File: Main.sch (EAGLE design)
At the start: 47 parts, among them IC1 LM75A, IC2 ADUM1400, IC3 74LS14N, Q1 IRF9530, U1 L298, U2 LM 1084 IT5,0, U3 LM 1084 IT3,3, U4 L298, X1 Motors, X2 PIRs, X3 Battery, X4 Ultra Sonics

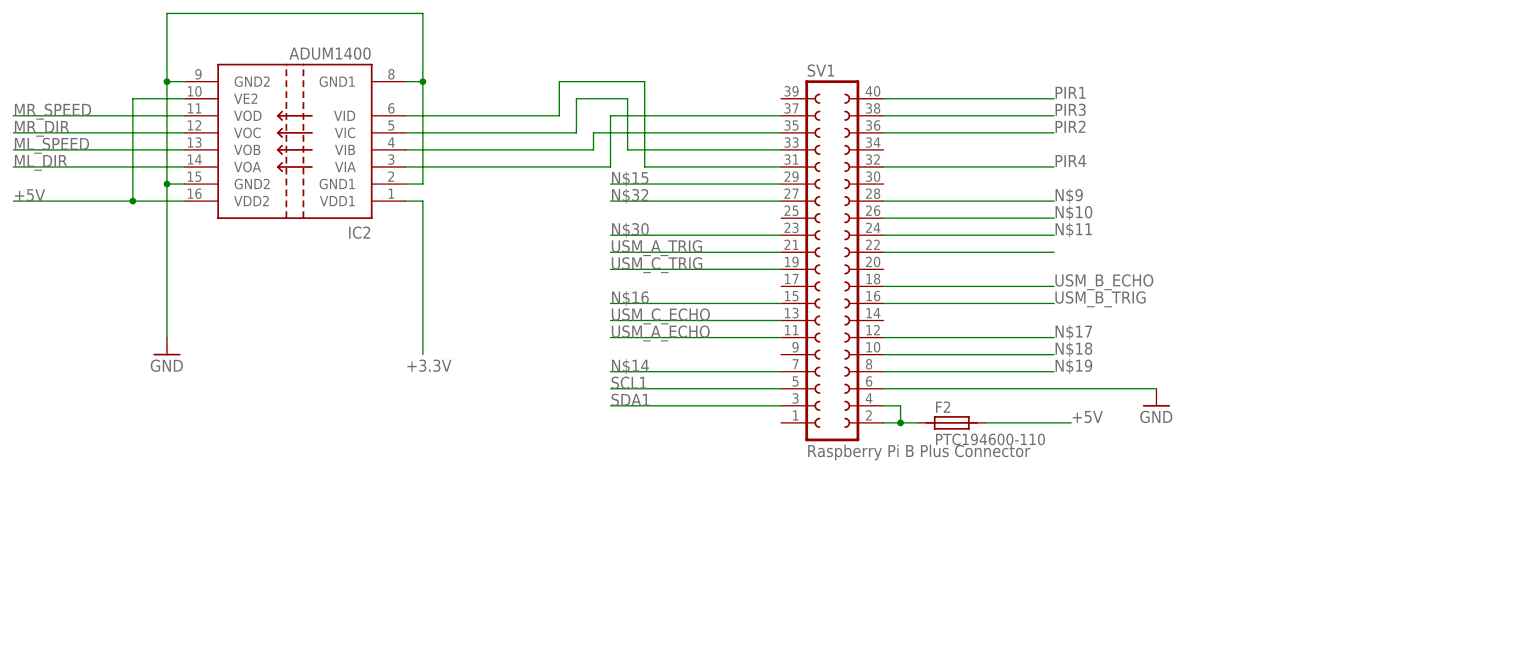
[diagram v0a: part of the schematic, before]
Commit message: playing with routes
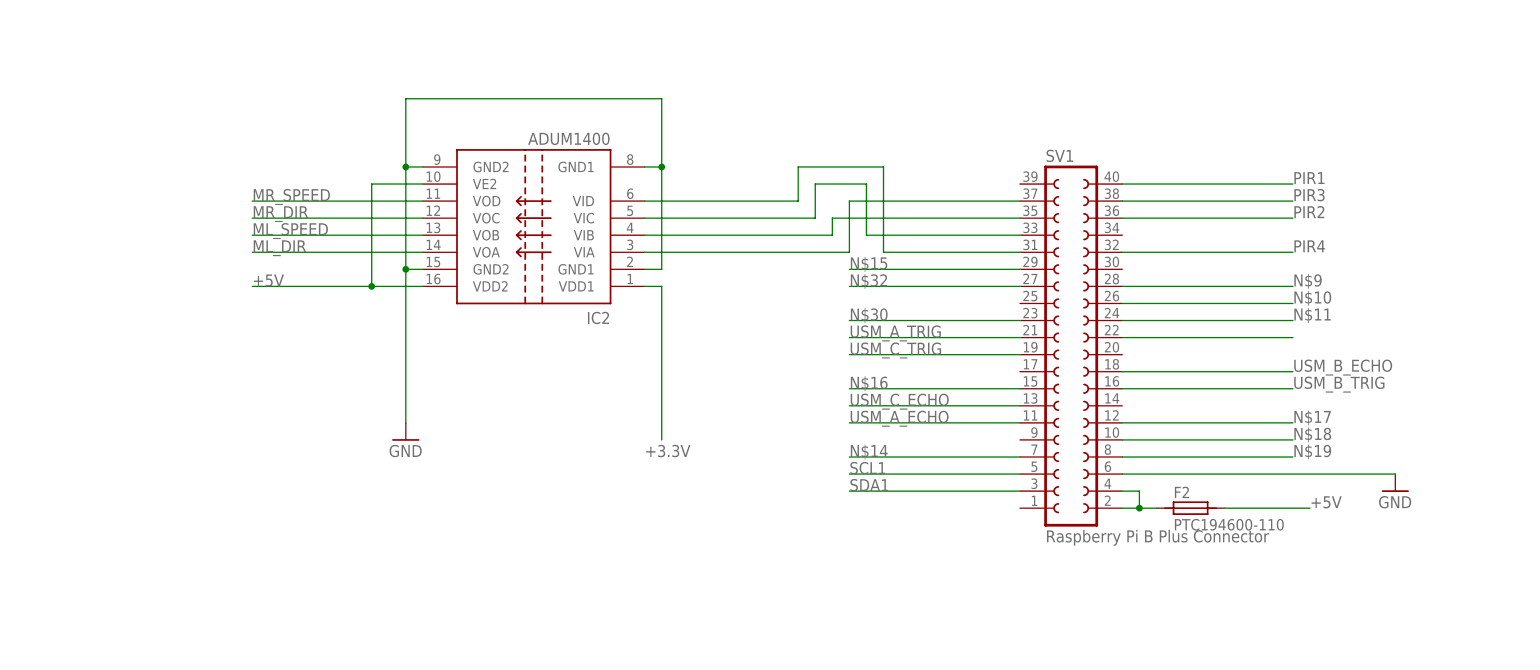
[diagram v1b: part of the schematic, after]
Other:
- moved on the sheet: F2, IC2, SV1
